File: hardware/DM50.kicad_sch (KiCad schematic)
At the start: 106 parts, among them J1 ST-LINK, J2 USB_C_Receptacle_USB2.0_14P, J4 Conn_01x04, Q1 MMBT3904, SW1 SW_SPST, SW10 BT_SMD, SW11 BT_SMD, SW12 BT_SMD, SW13 BT_SMD, SW14 BT_SMD, SW15 BT_SMD, SW16 BT_SMD, SW17 BT_SMD, SW18 BT_SMD, SW19 BT_SMD, SW2 BT_SMD, SW20 BT_SMD, SW21 BT_SMD, SW22 BT_SMD, SW23 BT_SMD, SW24 BT_SMD, SW25 BT_SMD, SW26 BT_SMD, SW27 BT_SMD, SW28 BT_SMD, SW29 BT_SMD, SW3 BT_SMD, SW30 BT_SMD, SW31 BT_SMD, SW32 BT_SMD, SW33 BT_SMD, SW34 BT_SMD, SW35 BT_SMD, SW36 BT_SMD, SW37 BT_SMD, SW38 BT_SMD, SW39 BT_SMD, SW4 BT_SMD, SW40 BT_SMD, SW41 BT_SMD, SW42 SW_SPST, SW43 BT_SMD, SW44 BT_SMD, SW45 BT_SMD, SW46 BT_SMD, SW47 BT_SMD, SW48 BT_SMD, SW49 BT_SMD, SW5 BT_SMD, SW50 BT_SMD, SW51 BT_SMD, SW52 BT_SMD, SW6 BT_SMD, SW7 BT_SMD, SW8 BT_SMD, SW9 BT_SMD, U1 EA_DOGL128X-6, U2 STM32U535CBT6, U3 AT25SF641, U4 USBLC6-2SC6, U5 ADP2108AUJ-3.3, U6 MCP73831-2-OT, Y1 32768

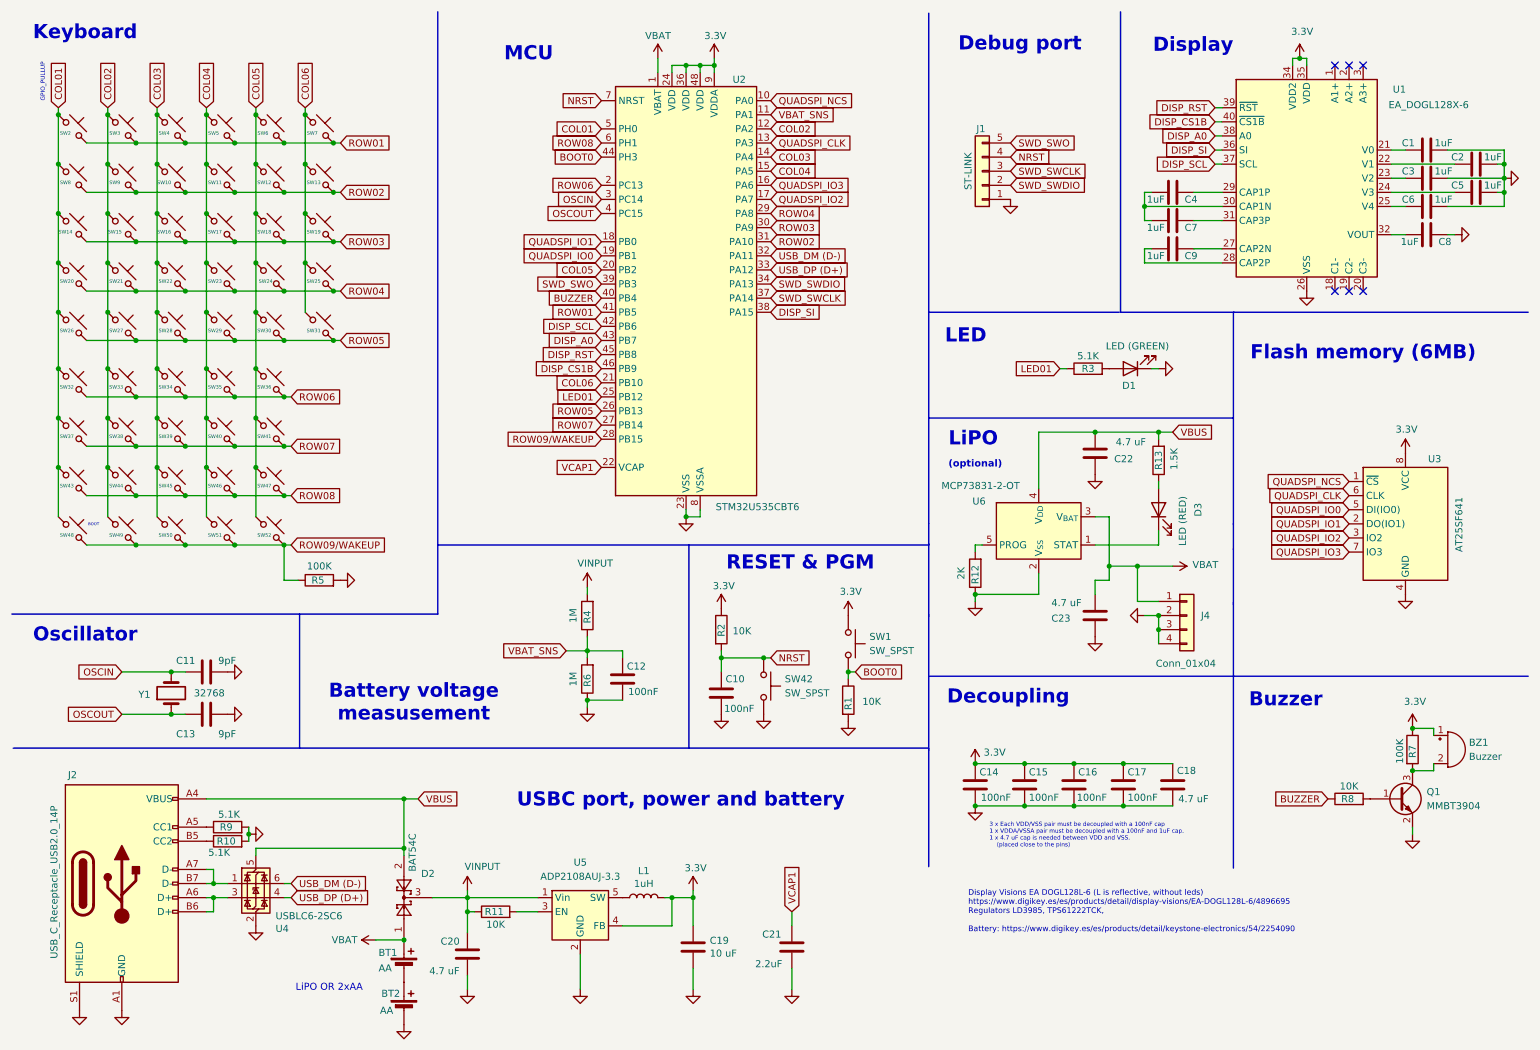
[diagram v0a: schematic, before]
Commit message: LiPO CONNECTOR
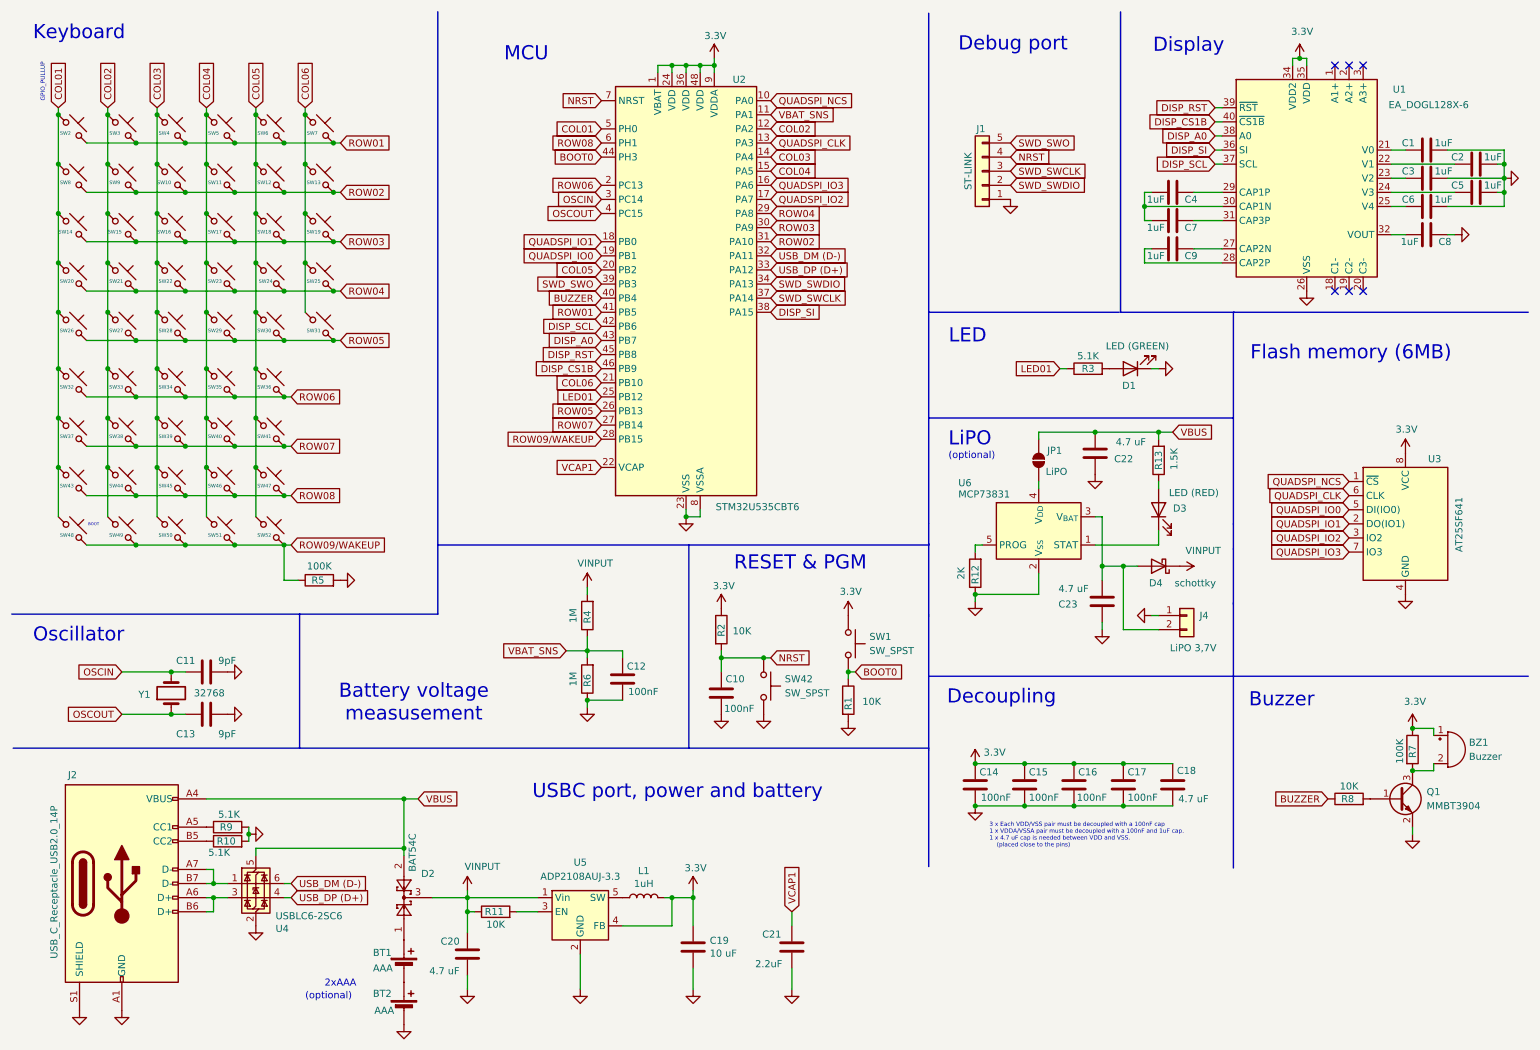
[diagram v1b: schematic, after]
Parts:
- added D4: schottky, Diode_SMD:D_SOD-323, symbol Device:D_Schottky
- added JP1: LiPO, Jumper:SolderJumper-2_P1.3mm_Bridged_RoundedPad1.0x1.5mm, symbol Jumper:SolderJumper_2_Open
- BT1, BT2: value AA -> AAA
- J4: value Conn_01x04 -> LiPO 3,7V; footprint DM50:CONN_S2B-ZR-SM4A-TFLFSN_JST -> DM50:CONN_S2B-PH-K-S_JST; symbol Connector_Generic:Conn_01x04 -> Connector_Generic:Conn_01x02
- U6: value MCP73831-2-OT -> MCP73831
- Y1: footprint Crystal:Crystal_SMD_MicroCrystal_CM9V-T1A-2Pin_1.6x1.0mm -> DM50:XTAL_ABS05-32.768KHZ-9-T
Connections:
- net 3.3V: now also U2.1 (VBAT)
- net GND: now also J4.1 (Pin_1); no longer J4.2 (Pin_2), J4.3 (Pin_3), J4.4 (Pin_4)
- net VBUS: now also JP1.2 (B); no longer U6.4 (V_{DD})
- net VINPUT: now also D4.1 (K)
- removed net VBAT: BT1.1 (+), C23.1, D2.1, J4.1 (Pin_1), U2.1 (VBAT), U6.3 (V_{BAT})
- new net: JP1.1 (A), U6.4 (V_{DD})
- new net: BT1.1 (+), D2.1
- new net: C23.1, D4.2 (A), J4.2 (Pin_2), U6.3 (V_{BAT})
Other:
- note added: "2xAAA"
- note removed: "Display Visions EA DOGL128L-6 (L is reflective, without leds) https://www.digikey.es/es/products/detail/display-visions/EA-DOGL128L-6/4896695 Regulators LD3985, TPS61222TCK, Battery: https://www.digikey.es/es/products/detail/keystone-electronics/54/2254090"
- note removed: "LiPO OR 2xAA"
- moved on the sheet: C23
